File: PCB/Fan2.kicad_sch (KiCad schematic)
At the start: 5 parts, among them J2 Conn_01x02, Q2 IRLML0030

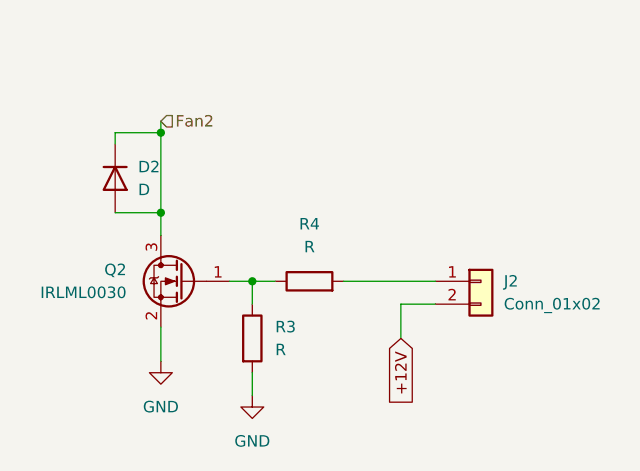
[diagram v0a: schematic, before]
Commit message: finished PCB
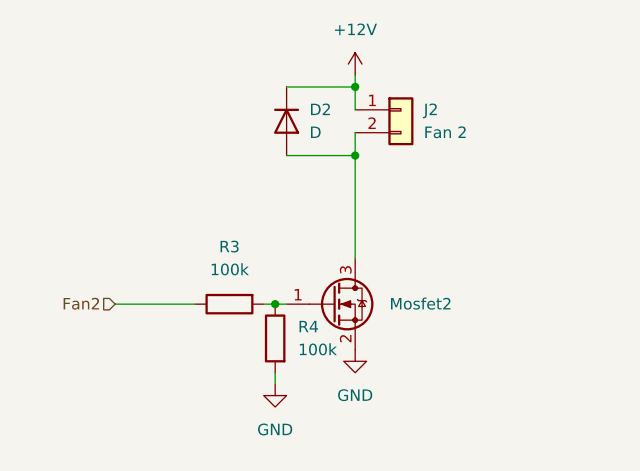
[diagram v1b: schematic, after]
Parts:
- removed Q2: IRLML0030, Package_TO_SOT_SMD:SOT-23, symbol Transistor_FET:IRLML0030
- added Mosfet2: IRLML0030, Package_TO_SOT_SMD:SOT-23, symbol Transistor_FET:IRLML0030
- J2: value Conn_01x02 -> Fan 2
- R3, R4: value R -> 100k
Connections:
- net +12V: now also D2.1 (K), J2.1 (Pin_1); no longer J2.2 (Pin_2)
- net Fan2: now also R3.1; no longer D2.1 (K), D2.2 (A)
- net GND: now also R4.2, Mosfet2.2 (S); no longer R3.2
- net at R4.1: now also R3.2, Mosfet2.1 (G); no longer R3.1
- new net: D2.2 (A), J2.2 (Pin_2), Mosfet2.3 (D)
